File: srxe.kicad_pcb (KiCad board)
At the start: 2 copper layers, 48.3 x 10.2 mm, 3 parts

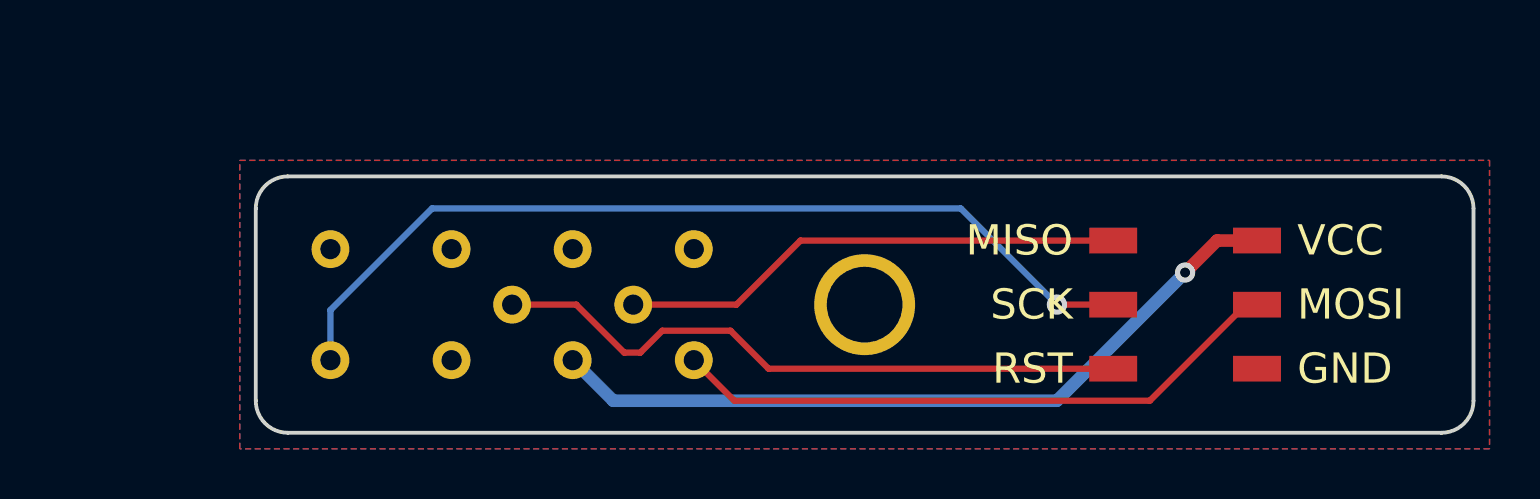
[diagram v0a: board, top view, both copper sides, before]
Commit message: align grid
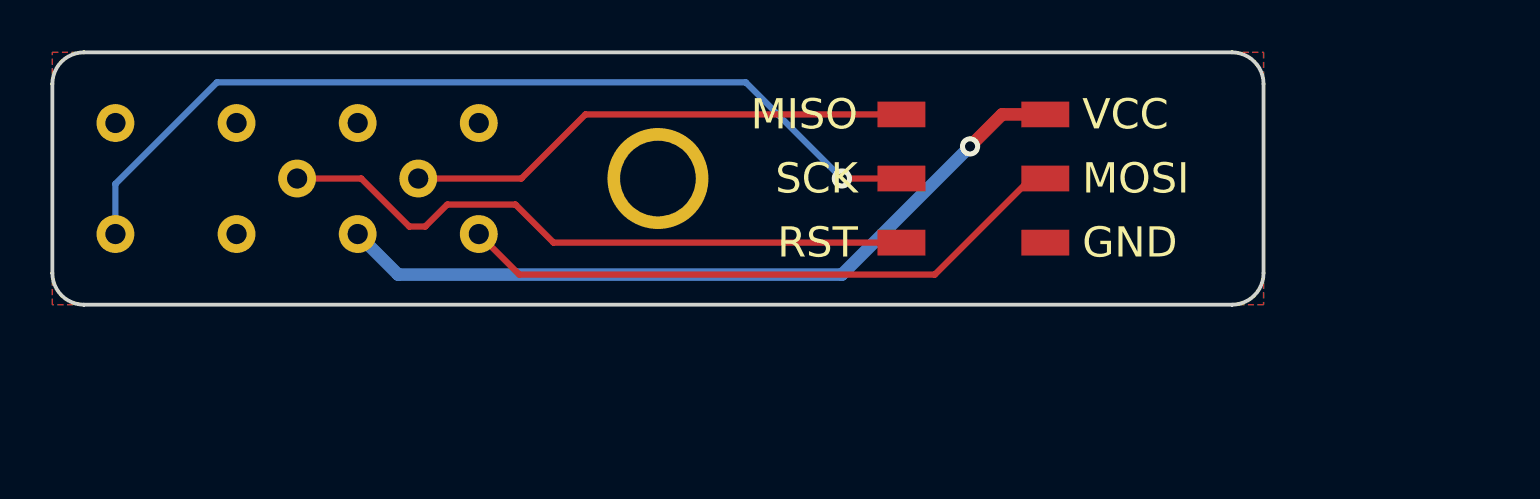
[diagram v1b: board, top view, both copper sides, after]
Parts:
- moved H1 9.88 mm to (149.7, 100.0)
- moved U$1 9.88 mm to (135.7, 100.0)
- moved JP2 9.77 mm to (162.5, 100.0)
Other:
- board size 48.3 x 10.2 mm -> 48 x 10 mm
